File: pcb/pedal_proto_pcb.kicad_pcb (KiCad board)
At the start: 2 copper layers, 90 x 70 mm, 36 parts, among them J1 100k_pot_1, J10 100k_pot_1_B, J11 100k_pot_1_C, J12 100k_pot_2_A, J13 100k_pot_2_B, J14 100k_pot_2_C, J15 250k_pot_1_A, J16 250k_pot_1_B, J17 250k_pot_1_C, J18 250k_pot_2_A, J19 250k_pot_2_B, J2 100k_pot_2, J20 250k_pot_2_C, J21 stomp_1_A, J22 stomp_1_B, J23 stomp_1_C, J24 stomp_2_A, J25 stomp_2_B, J26 stomp_2_C, J27 stomp_3_A, J28 stomp_3_B, J29 stomp_2_C, J3 250k_pot_1, J30 switch_A, J31 switch_B, J32 switch_C, J33 GND, J34 VDD, J35 LED-, J36 LED+, J4 250k_pot_2, J5 stomp, J6 switch, J7 power, J8 LED, J9 100k_pot_1_A

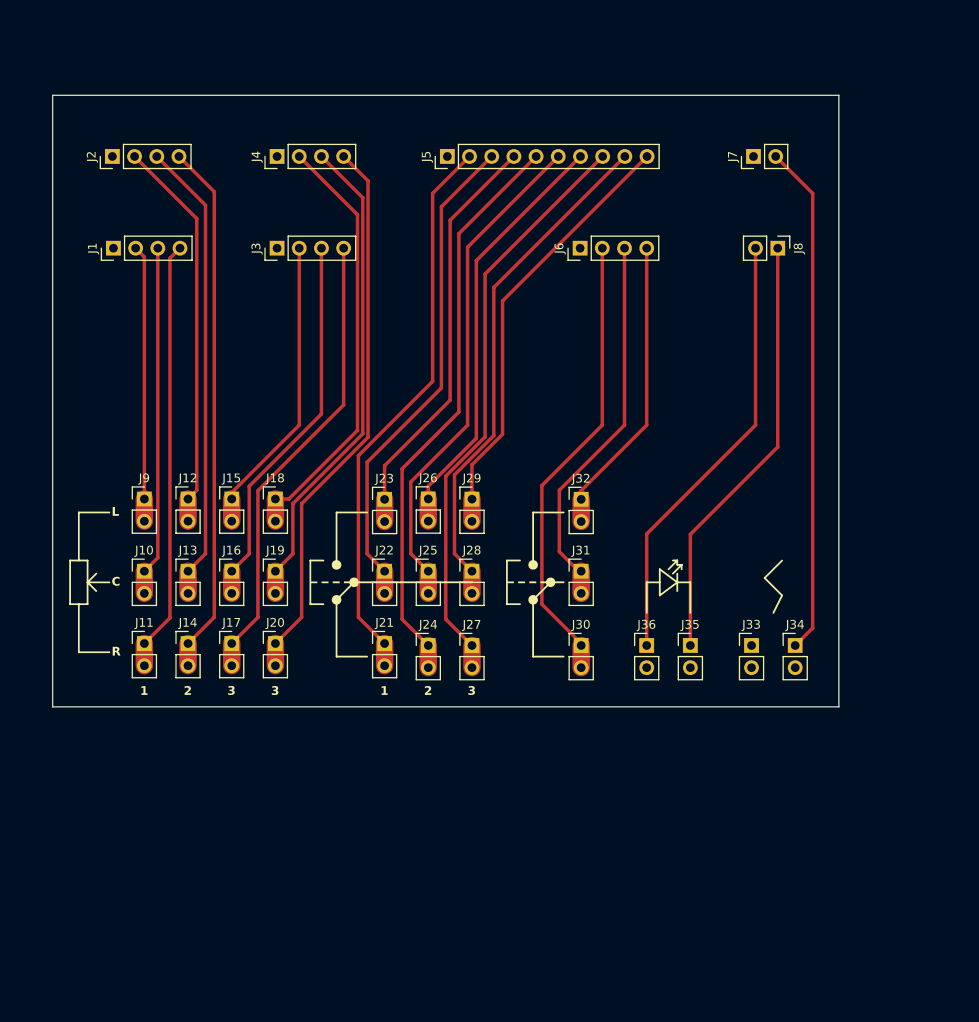
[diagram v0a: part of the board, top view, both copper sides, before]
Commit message: feat: updated pcb
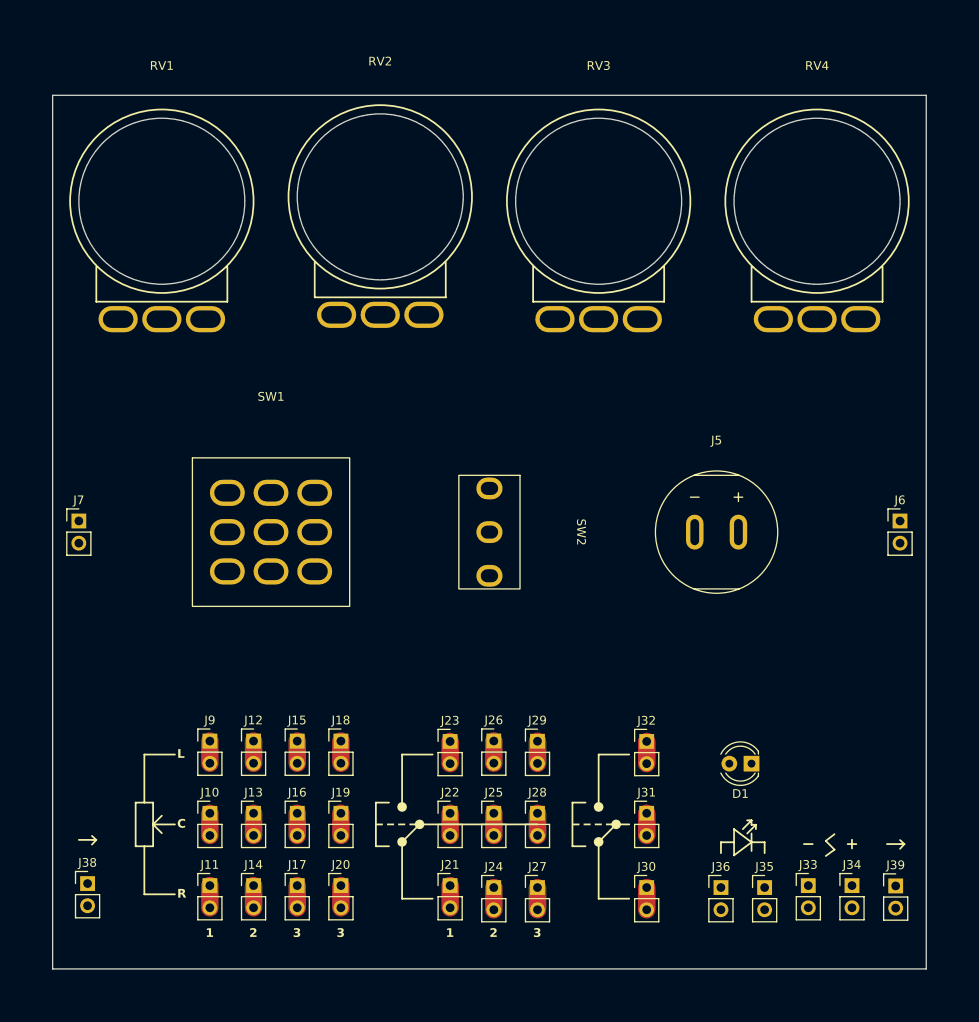
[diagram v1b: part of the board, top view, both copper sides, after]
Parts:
- removed J1: 100k_pot_1, Connector_PinHeader_2.54mm:PinHeader_1x04_P2.54mm_Vertical
- removed J2: 100k_pot_2, Connector_PinHeader_2.54mm:PinHeader_1x04_P2.54mm_Vertical
- removed J3: 250k_pot_1, Connector_PinHeader_2.54mm:PinHeader_1x04_P2.54mm_Vertical
- removed J4: 250k_pot_2, Connector_PinHeader_2.54mm:PinHeader_1x04_P2.54mm_Vertical
- removed J8: LED, Connector_PinHeader_2.54mm:PinHeader_1x02_P2.54mm_Vertical
- added D1: LED, LED_THT:LED_D4.0mm, F.Cu at (199.5, 131.0)
- added J38: input, Connector_PinHeader_2.54mm:PinHeader_1x02_P2.54mm_Vertical, F.Cu at (123.5, 144.7)
- added J39: output, Connector_PinHeader_2.54mm:PinHeader_1x02_P2.54mm_Vertical, F.Cu at (216.0, 145.0)
- added RV1: 100k_Potentiometer, Additional_Switches:Lug_Pot, F.Cu at (132.0, 51.6)
- added RV2: 100k_Potentiometer, Additional_Switches:Lug_Pot, F.Cu at (157.0, 51.1)
- added RV3: 250k_Potentiometer, Additional_Switches:Lug_Pot, F.Cu at (182.0, 51.6)
- added RV4: 250k_Potentiometer, Additional_Switches:Lug_Pot, F.Cu at (207.0, 51.6)
- added SW1: SW_3PDT, Additional_Switches:3PDT, F.Cu at (144.5, 89.5)
- added SW2: SW_SPDT, Additional_Switches:SPDT, F.Cu at (179.5, 104.5)
- J10: value 100k_pot_1_B -> RV1_2
- J11: value 100k_pot_1_C -> RV1_1
- J12: value 100k_pot_2_A -> RV2_3
- J13: value 100k_pot_2_B -> RV2_2
- J14: value 100k_pot_2_C -> RV2_1
- J15: value 250k_pot_1_A -> RV3_3
- J16: value 250k_pot_1_B -> RV3_2
- J17: value 250k_pot_1_C -> RV3_1
- J18: value 250k_pot_2_A -> RV4_3
- J19: value 250k_pot_2_B -> RV4_2
- J20: value 250k_pot_2_C -> RV4_1
- J21: value stomp_1_A -> stomp_A_1
- J22: value stomp_1_B -> stomp_A_2
- J23: value stomp_1_C -> stomp_A_3
- J24: value stomp_2_A -> stomp_B_1
- J25: value stomp_2_B -> stomp_B_2
- J26: value stomp_2_C -> stomp_B_3
- J27: value stomp_3_A -> stomp_C_1
- J28: value stomp_3_B -> stomp_C_2
- J29: value stomp_2_C -> stomp_C_3
- J30: value switch_A -> switch_1
- J31: value switch_B -> switch_2
- J32: value switch_C -> switch_3
- J5: value stomp -> Jack-DC; footprint Connector_PinHeader_2.54mm:PinHeader_1x10_P2.54mm_Vertical -> Additional_Connectors:Barrel_Plug_5.5mmx2.1mm
- J6: value switch -> Barrel_Jack_Output; footprint Connector_PinHeader_2.54mm:PinHeader_1x04_P2.54mm_Vertical -> Connector_PinHeader_2.54mm:PinHeader_1x02_P2.54mm_Vertical
- J7: value power -> Barrel_Jack_Input
- J9: value 100k_pot_1_A -> RV1_3
- moved J7 87.8 mm to (122.5, 103.2), turned to 0 degrees
- moved J6 48.1 mm to (216.5, 103.2), turned to 0 degrees
- moved J5 45.2 mm to (195.5, 94.5), turned to 0 degrees
- moved J35 29.0 mm to (201.0, 145.2)
- moved J36 29.0 mm to (196.0, 145.2)
- moved J10 28.7 mm to (137.5, 136.7)
- moved J11 28.7 mm to (137.5, 145.0)
- moved J13 28.7 mm to (142.5, 136.7)
- moved J14 28.7 mm to (142.5, 145.0)
- moved J16 28.7 mm to (147.5, 136.7)
- moved J17 28.7 mm to (147.5, 145.0)
- moved J19 28.7 mm to (152.5, 136.7)
- moved J20 28.7 mm to (152.5, 145.0)
- moved J21 28.7 mm to (165.0, 145.0)
- moved J22 28.7 mm to (165.0, 136.7)
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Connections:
- J34 pad 1: /VDD -> Net-(J34-Pin_1)
- J34 pad 2: /VDD -> Net-(J34-Pin_1)
- J5 pad 1: 0 -> Net-(J34-Pin_1)
- J5 pad 2: Net-(J21-Pin_1) -> 0
- J6 pad 2: Net-(J30-Pin_1) -> Net-(J39-Pin_1)
- J7 pad 2: /VDD -> Net-(J38-Pin_1)
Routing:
- net Net-(J27-Pin_1): track 67.2 -> 2.54 mm
- net Net-(J24-Pin_1): track 66.1 -> 2.54 mm
- net Net-(J21-Pin_1): track 64.8 -> 2.54 mm
- net Net-(J20-Pin_1): track 63.8 -> 2.54 mm
- net Net-(J14-Pin_1): track 61.2 -> 2.54 mm
- net /VDD: track 58.6 -> 0.00 mm
- net Net-(J28-Pin_1): track 58.9 -> 2.54 mm
- net Net-(J25-Pin_1): track 57.8 -> 2.54 mm
- net Net-(J22-Pin_1): track 57.2 -> 2.54 mm
- net Net-(J19-Pin_1): track 56.1 -> 2.54 mm
- net Net-(D1-A): track 50.6 -> 0.00 mm
- net Net-(J13-Pin_1): track 53.2 -> 2.54 mm
- net Net-(J17-Pin_1): track 53.1 -> 2.54 mm
- net Net-(J30-Pin_1): track 52.7 -> 2.54 mm
- net Net-(D1-K): track 49.6 -> 0.00 mm
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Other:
- board size 90 x 70 mm -> 100 x 100 mm
